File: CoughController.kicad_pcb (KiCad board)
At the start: 2 copper layers, 144 x 100 mm, 59 parts, among them J1 カフＳＷ１, J10 音声入力, J11 音声出力, J12 DI-2, J13 DO-2, J14 CD1/CD2, J15 CF/MD, J16 IN1/IN2, J17 IN3/IN4, J2 カフＳＷ２, J3 カフＳＷ３, J4 カフＳＷ４, J5 カフＳＷ５, J6 電源入力, J7 電源出力, J8 DI-1, J9 DO-1, K1 G6A-274P-ST-US DC12, K2 G6A-274P-ST-US DC12, U1 TLP627-2, U2 TLP627-2, U3 TLP627-2, U4 TLP627-2, U5 TLP627-2, U6 TLP627-2, U7 TLP627-2, U8 TLP627-2

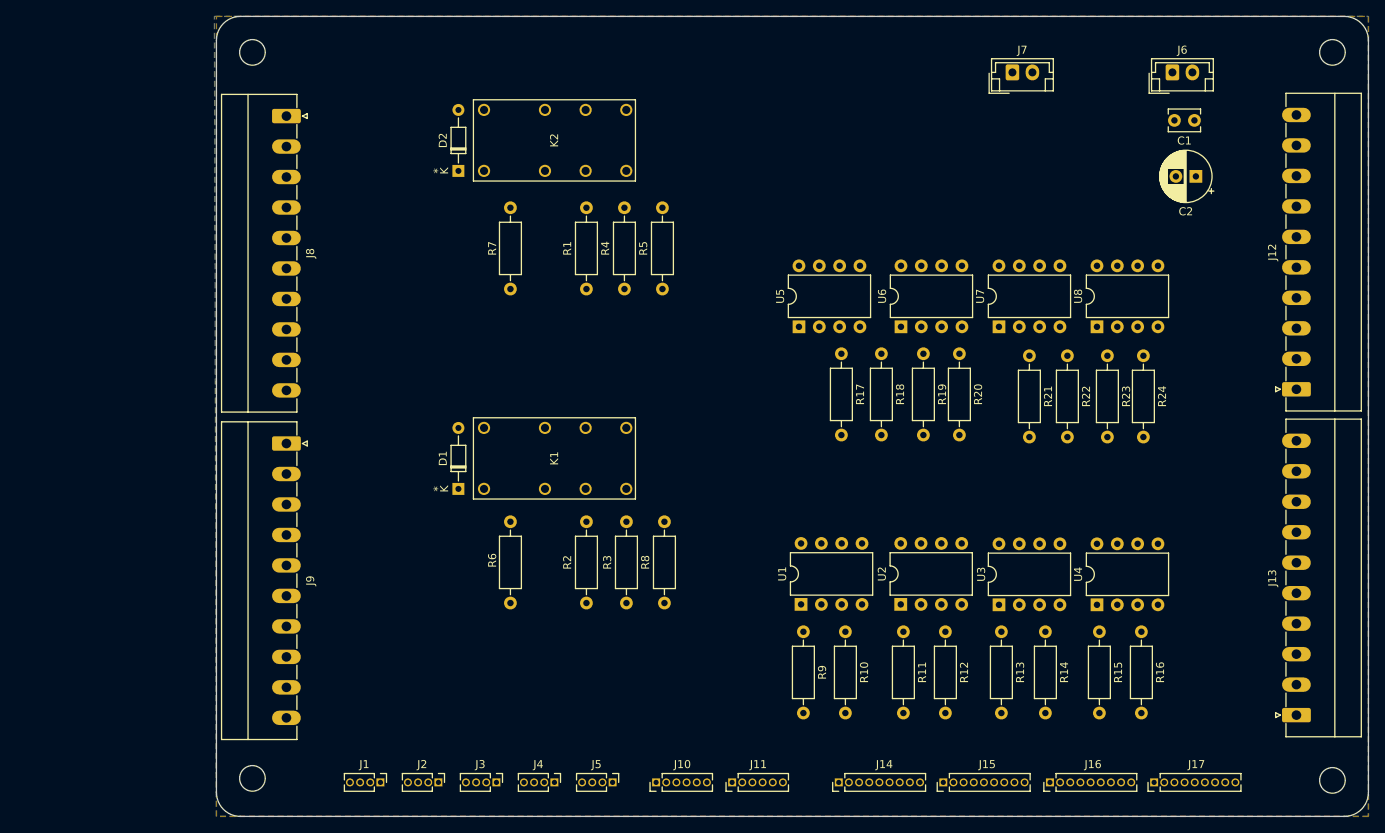
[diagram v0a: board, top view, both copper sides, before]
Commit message: カフコントローラ
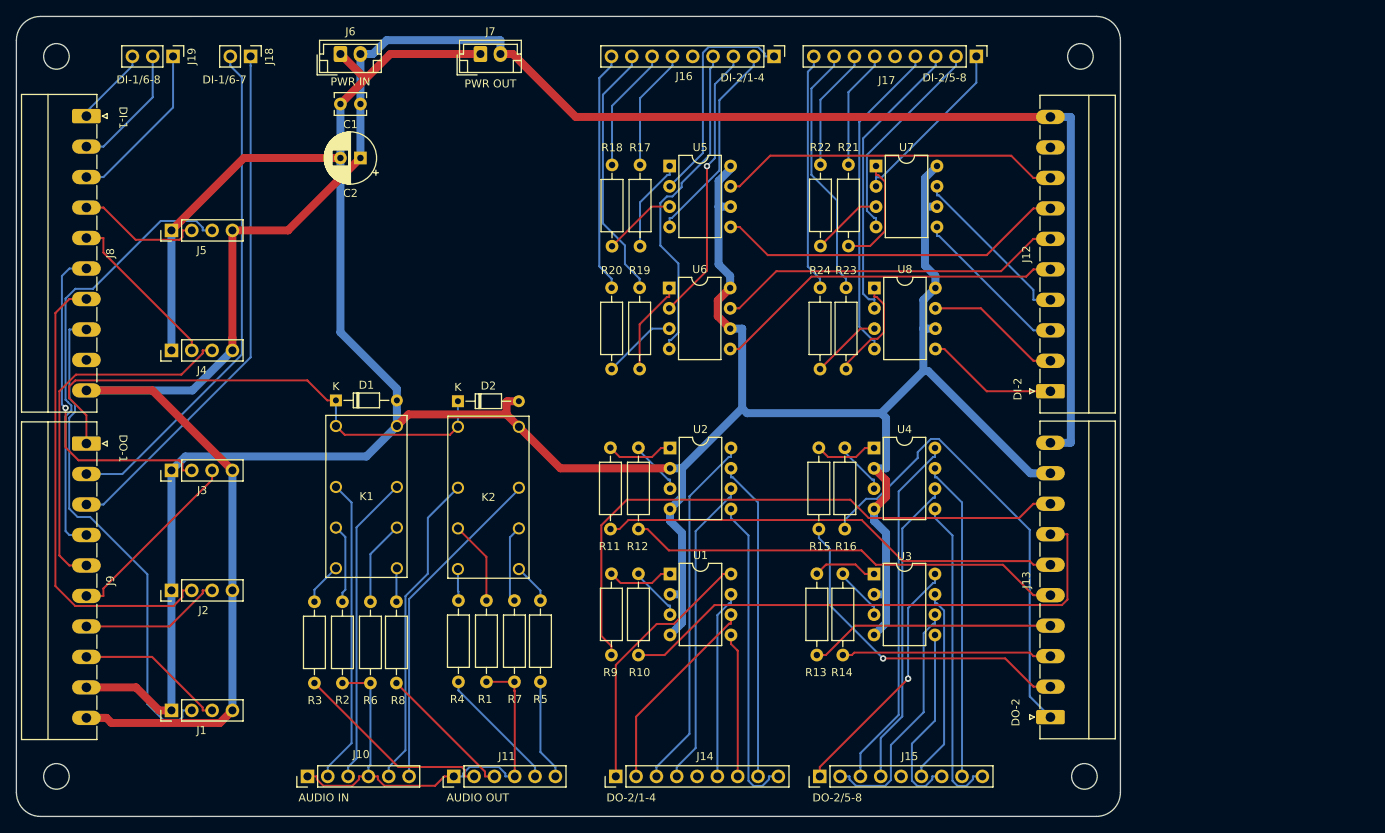
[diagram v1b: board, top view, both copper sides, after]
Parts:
- added J18: Out, Connector_PinHeader_2.54mm:PinHeader_1x02_P2.54mm_Vertical, F.Cu at (79.3, 55.0)
- added J19: In, Connector_PinHeader_2.54mm:PinHeader_1x03_P2.54mm_Vertical, F.Cu at (69.6, 55.0)
- J1: value カフＳＷ１ -> SW1; footprint Connector_PinHeader_1.27mm:PinHeader_1x04_P1.27mm_Vertical -> Connector_PinHeader_2.54mm:PinHeader_1x04_P2.54mm_Vertical
- J10: value 音声入力 -> AUDIO_IN; footprint Connector_PinHeader_1.27mm:PinHeader_1x06_P1.27mm_Vertical -> Connector_PinHeader_2.54mm:PinHeader_1x06_P2.54mm_Vertical
- J11: value 音声出力 -> AUDIO_OUT; footprint Connector_PinHeader_1.27mm:PinHeader_1x06_P1.27mm_Vertical -> Connector_PinHeader_2.54mm:PinHeader_1x06_P2.54mm_Vertical
- J14, J15, J16, J17: footprint Connector_PinHeader_1.27mm:PinHeader_1x09_P1.27mm_Vertical -> Connector_PinHeader_2.54mm:PinHeader_1x09_P2.54mm_Vertical
- J2: value カフＳＷ２ -> SW2; footprint Connector_PinHeader_1.27mm:PinHeader_1x04_P1.27mm_Vertical -> Connector_PinHeader_2.54mm:PinHeader_1x04_P2.54mm_Vertical
- J3: value カフＳＷ３ -> SW3; footprint Connector_PinHeader_1.27mm:PinHeader_1x04_P1.27mm_Vertical -> Connector_PinHeader_2.54mm:PinHeader_1x04_P2.54mm_Vertical
- J4: value カフＳＷ４ -> SW4; footprint Connector_PinHeader_1.27mm:PinHeader_1x04_P1.27mm_Vertical -> Connector_PinHeader_2.54mm:PinHeader_1x04_P2.54mm_Vertical
- J5: value カフＳＷ５ -> SW5; footprint Connector_PinHeader_1.27mm:PinHeader_1x04_P1.27mm_Vertical -> Connector_PinHeader_2.54mm:PinHeader_1x04_P2.54mm_Vertical
- J6: value 電源入力 -> PWR_IN
- J7: value 電源出力 -> PWR_OUT
- moved H3 183.4 mm to (55.0, 145.0)
- moved C2 104.5 mm to (93.0, 67.7)
- moved C1 104.3 mm to (93.0, 61.0)
- moved J6 104.0 mm to (90.5, 54.7)
- moved H2 103.5 mm to (183.0, 55.0)
- moved J16 97.1 mm to (144.7, 55.0), turned to -90 degrees
- moved H1 93.5 mm to (55.0, 55.0)
- moved J17 93.4 mm to (170.0, 55.0), turned to -90 degrees
- moved J5 88.3 mm to (69.4, 76.8), turned to 90 degrees
- moved J4 72.2 mm to (69.4, 91.8), turned to 90 degrees
- moved J7 66.5 mm to (108.0, 54.7)
- moved K2 58.7 mm to (112.8, 118.9), turned to 0 degrees
- moved J3 56.3 mm to (69.4, 106.8), turned to 90 degrees
- moved R4 53.3 mm to (105.2, 133.2)
- moved R5 51.4 mm to (115.5, 133.2)
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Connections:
- J12 pad 10: COM2 -> COM0
- J13 pad 10: COM2 -> COM0
- J13 pad 9: MCOM3 -> MCOM1
- J8 pad 1: unconnected-(J8-Pin_1-Pad1) -> Net-(J19-Pin_3)
- J8 pad 2: unconnected-(J8-Pin_2-Pad2) -> Net-(J19-Pin_2)
- J8 pad 3: unconnected-(J8-Pin_3-Pad3) -> Net-(J19-Pin_1)
- J9 pad 2: unconnected-(J9-Pin_2-Pad2) -> Net-(J18-Pin_2)
- J9 pad 3: unconnected-(J9-Pin_3-Pad3) -> Net-(J18-Pin_1)
- U1 pad 2: MCOM3 -> MCOM1
- U1 pad 4: MCOM3 -> MCOM1
- U2 pad 2: MCOM3 -> MCOM1
- U2 pad 4: MCOM3 -> MCOM1
- U3 pad 2: MCOM3 -> MCOM1
- U3 pad 4: MCOM3 -> MCOM1
- U4 pad 2: MCOM3 -> MCOM1
- U4 pad 4: MCOM3 -> MCOM1
- U5 pad 6: MCOM3 -> MCOM1
- U5 pad 8: MCOM3 -> MCOM1
- U6 pad 6: MCOM3 -> MCOM1
- U6 pad 8: MCOM3 -> MCOM1
- U7 pad 6: MCOM3 -> MCOM1
- U7 pad 8: MCOM3 -> MCOM1
- U8 pad 6: MCOM3 -> MCOM1
- U8 pad 8: MCOM3 -> MCOM1
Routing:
- net MCOM1: track 0.00 -> 402.8 mm
- net COM0: track 0.00 -> 277.4 mm
- net Net-(J13-Pin_8): track 0.00 -> 75.9 mm
- net Net-(J13-Pin_7): track 0.00 -> 66.8 mm
- net Net-(J18-Pin_1): track 0.00 -> 65.8 mm
- net RY_POW: track 0.00 -> 65.2 mm
- net Net-(J18-Pin_2): track 0.00 -> 63.5 mm
- net Net-(J1-Pin_2): track 0.00 -> 61.8 mm
- net Net-(J10-Pin_1): track 0.00 -> 60.5 mm
- net Net-(J2-Pin_2): track 0.00 -> 58.1 mm
- net Net-(J13-Pin_1): track 0.00 -> 58.1 mm
- net Net-(J13-Pin_6): track 0.00 -> 57.8 mm
- net Net-(J5-Pin_3): track 0.00 -> 55.5 mm
- net Net-(J13-Pin_5): track 0.00 -> 54.9 mm
- net Net-(J4-Pin_3): track 0.00 -> 45.9 mm
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- removed copper zone on B.Cu, net MCOM1
- removed copper zone on F.Cu, net MCOM1
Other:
- board size 144 x 100 mm -> 138 x 100 mm
- board text added: "AUDIO IN"
- board text added: "AUDIO OUT"
- board text added: "DI-1"
- board text added: "DI-1/6-7"
- board text added: "DI-1/6-8"
- board text added: "DI-2"
- board text added: "DI-2/1-4"
- board text added: "DI-2/5-8"
- board text added: "DO-1"
- board text added: "DO-2"
- board text added: "DO-2/1-4"
- board text added: "DO-2/5-8"
- board text added: "PWR IN"
- board text added: "PWR OUT"
